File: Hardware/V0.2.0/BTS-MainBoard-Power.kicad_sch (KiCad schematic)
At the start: 33 parts, among them J1 +12VIn, J12 Conn_01x02, J13 Conn_01x02, J14 Conn_01x02, J15 Conn_01x02, J16 Conn_01x02, J17 Conn_01x02, J18 Conn_01x02, J19 Conn_01x02, J2 GNDIn, J3 Conn_01x07, Q1 Q_NMOS_DGS, U1 LM5109BMA, U2 LM5109BMA

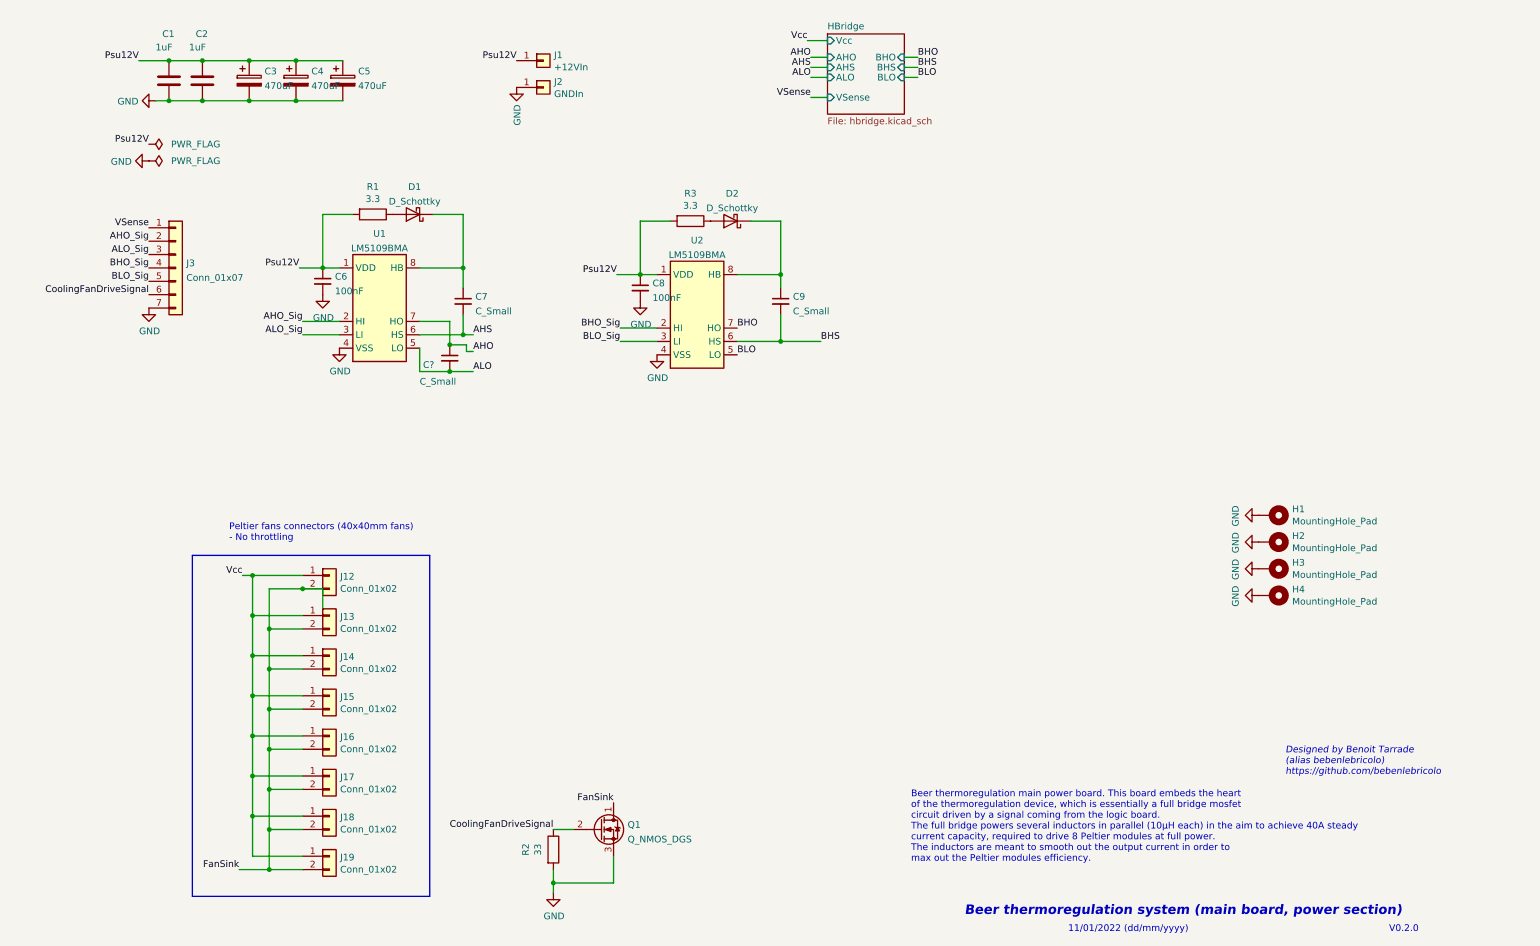
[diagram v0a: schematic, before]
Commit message: Started first routing steps
Signed-off-by: bebenlebricolo <benoittarrade@hotmail.fr>
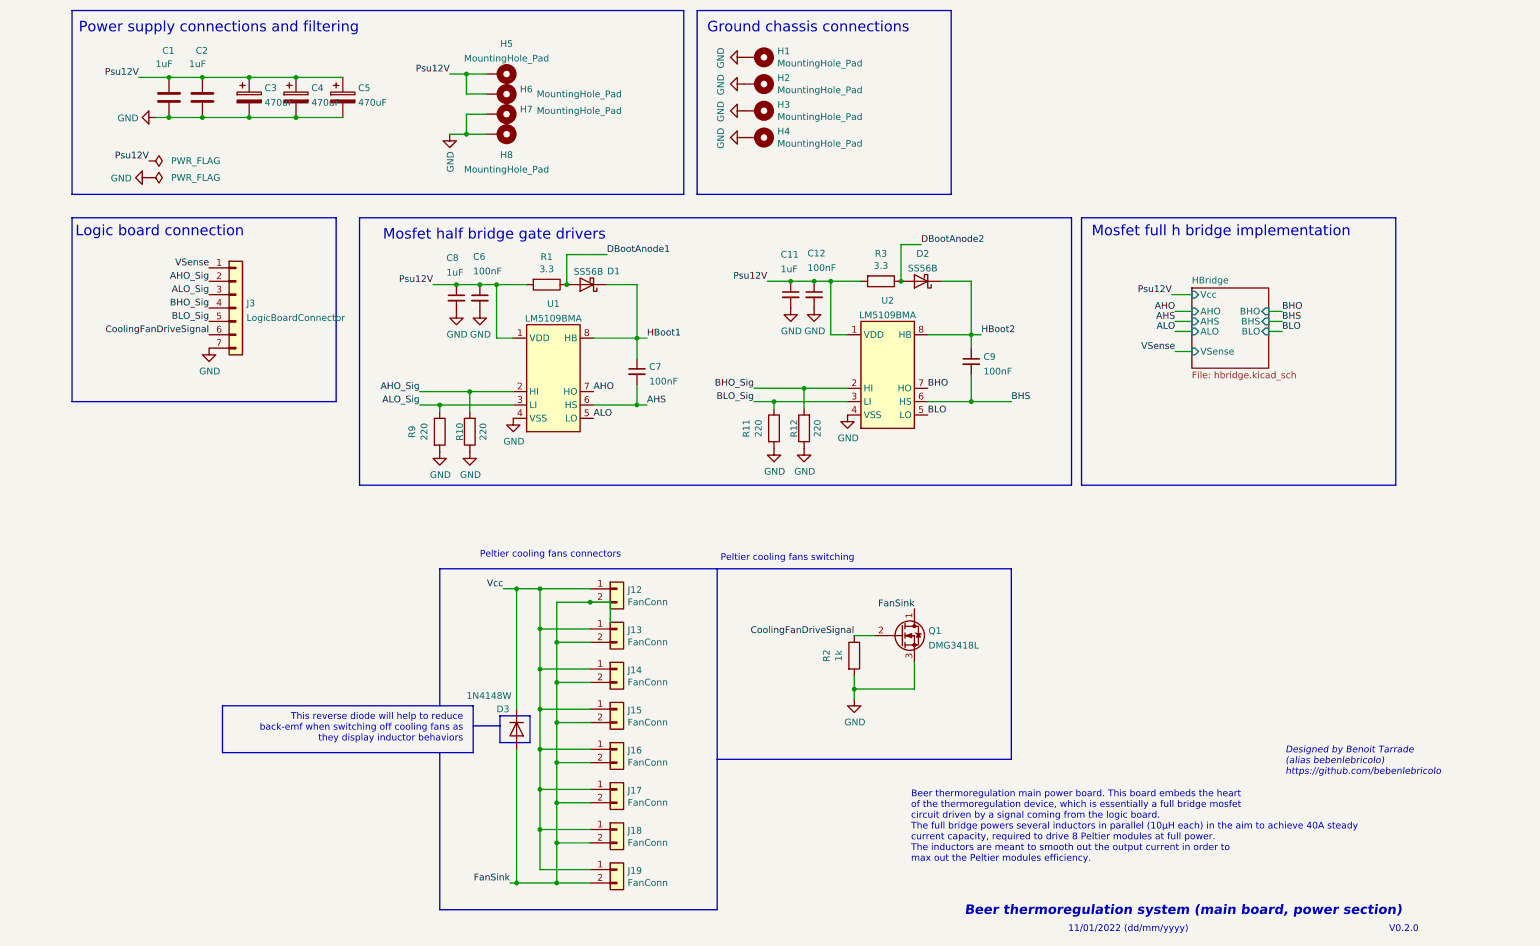
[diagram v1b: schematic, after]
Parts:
- removed C?: C_Small, symbol Device:C_Small
- removed J1: +12VIn, BTS-MainBoard-Power:Power_Solder_Pad_7x15mm, symbol Connector_Generic:Conn_01x01
- removed J2: GNDIn, BTS-MainBoard-Power:Power_Solder_Pad_7x15mm, symbol Connector_Generic:Conn_01x01
- added C11: 1uF, Capacitor_SMD:C_1206_3216Metric_Pad1.33x1.80mm_HandSolder, symbol Device:C_Small
- added C12: 100nF, Capacitor_SMD:C_1206_3216Metric_Pad1.33x1.80mm_HandSolder, symbol Device:C_Small
- added D3: 1N4148W, Diode_SMD:D_SOD-123, symbol Diode:1N4148W
- added H5, H6, H7, H8: MountingHole_Pad, MountingHole:MountingHole_3mm_Pad_Via, symbol Mechanical:MountingHole_Pad
- added R10, R11, R12, R9: 220, Resistor_SMD:R_1206_3216Metric_Pad1.30x1.75mm_HandSolder, symbol Device:R
- C7, C9: value C_Small -> 100nF; footprint (none) -> Capacitor_SMD:C_1206_3216Metric_Pad1.33x1.80mm_HandSolder
- C8: value 100nF -> 1uF
- D1, D2: value D_Schottky -> SS56B; footprint (none) -> BTS-MainBoard-Power:SS56B
- H1, H2, H3, H4: footprint MountingHole:MountingHole_4mm_Pad_TopOnly -> MountingHole:MountingHole_4mm_Pad_Via
- J12, J13, J14, J15, J16, J17, J18, J19: value Conn_01x02 -> FanConn; footprint Connector_PinHeader_2.54mm:PinHeader_1x02_P2.54mm_Vertical_SMD_Pin1Left -> Connector_PinSocket_2.54mm:PinSocket_1x02_P2.54mm_Vertical
- J3: value Conn_01x07 -> LogicBoardConnector; footprint (none) -> Connector_PinHeader_2.54mm:PinHeader_1x07_P2.54mm_Vertical
- Q1: value Q_NMOS_DGS -> DMG3418L; footprint (none) -> Package_TO_SOT_SMD:SOT-23
- R2: value 33 -> 1k
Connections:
- net AHO_Sig: now also R10.2
- net ALO_Sig: now also R9.1
- net BHO_Sig: now also R12.2
- net BLO_Sig: now also R11.1
- net FanSink: now also D3.2 (A)
- net GND: now also C11.2, C12.2, H7.1, H8.1, R10.1, R11.2, R12.1, R9.2
- net Psu12V: now also C11.1, C12.1, H5.1, H6.1
- net Vcc: now also D3.1 (K)
- net HBoot2: now reaches C9.1, D2.1 (K), U2.8 (HB)
- net DBootAnode1: now reaches D1.2 (A), R1.1
- net HBoot1: now reaches C7.1, D1.1 (K), U1.8 (HB)
- net DBootAnode2: now reaches D2.2 (A), R3.1
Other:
- note added: "Ground chassis connections"
- note added: "Logic board connection"
- note added: "Mosfet full h bridge implementation"
- note added: "Mosfet half bridge gate drivers"
- note added: "Peltier cooling fans connectors"
- note added: "Peltier cooling fans switching"
- note added: "Power supply connections and filtering"
- note added: "This reverse diode will help to reduce back-emf when switching off cooling fans as they display inductor behaviors"
- note removed: "Peltier fans connectors (40x40mm fans) - No throttling"
- moved on the sheet: C1, C2, C3, C4, C5, C6, C7, C9, D1, H1, H2, H3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
